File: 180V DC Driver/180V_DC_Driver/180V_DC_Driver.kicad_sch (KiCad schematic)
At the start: 14 parts, among them IC1 TLP250_F_, J1 DC_In, J2 DC_Out, J3 Logic_In, J4 12V_In, Q1 IRFP460PBF

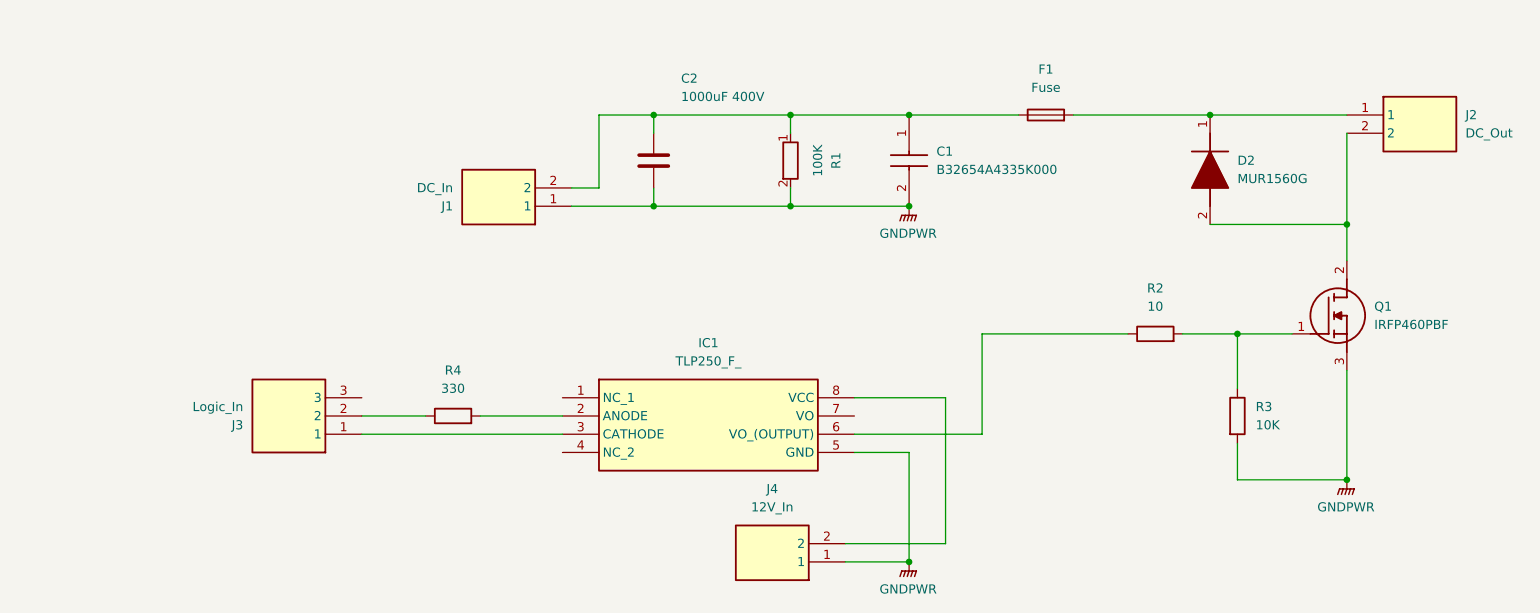
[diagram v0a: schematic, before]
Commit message: c2.06
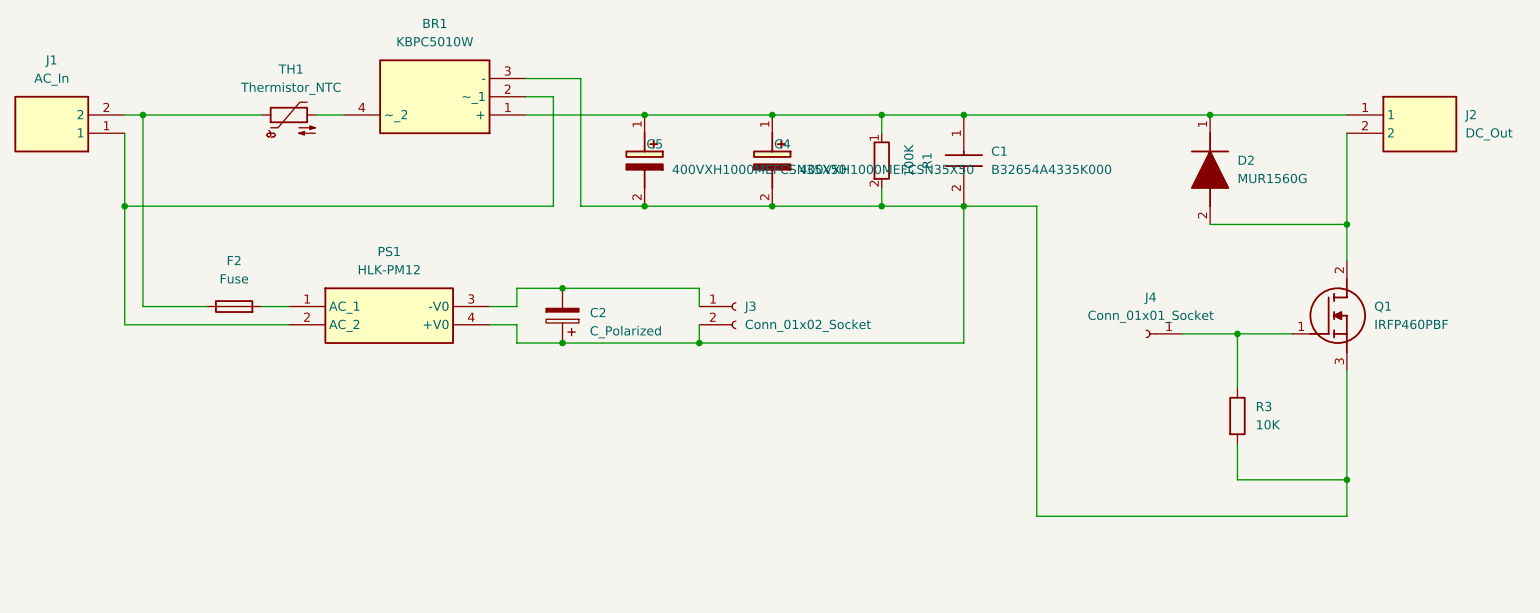
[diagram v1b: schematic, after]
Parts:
- removed C2: 1000uF 400V, symbol Device:C
- removed F1: Fuse, symbol Device:Fuse
- removed IC1: TLP250_F_, DIP762W60P254L966H485Q8N, symbol SamacSys_Parts:TLP250_F_
- removed J3: Logic_In, HDRV3W64P0X254_1X3_762X254X869P, symbol SamacSys_Parts:61300311121
- removed J4: 12V_In, 1935161, symbol SamacSys_Parts:1935161
- removed R2: 10, symbol Device:R
- removed R4: 330, symbol Device:R
- added BR1: KBPC5010W, Diode_THT:Diode_Bridge_28.6x28.6x7.3mm_P18.0mm_P11.6mm, symbol SamacSys_Parts:KBPC5010W
- added C2: C_Polarized, Capacitor_THT:CP_Radial_D6.3mm_P2.50mm, symbol Device:C_Polarized
- added C4, C5: 400VXH1000MEFCSN35X50, Capacitor_THT:CP_Radial_D35.0mm_P10.00mm_SnapIn, symbol SamacSys_Parts:400VXH1000MEFCSN35X50
- added F2: Fuse, Connector_PinHeader_2.54mm:PinHeader_1x02_P2.54mm_Vertical, symbol Device:Fuse
- added J3: Conn_01x02_Socket, Connector_PinHeader_2.54mm:PinHeader_1x02_P2.54mm_Vertical, symbol Connector:Conn_01x02_Socket
- added J4: Conn_01x01_Socket, Connector_PinHeader_2.54mm:PinHeader_1x01_P2.54mm_Vertical, symbol Connector:Conn_01x01_Socket
- added PS1: HLK-PM12, Converter_ACDC:Converter_ACDC_Hi-Link_HLK-PMxx, symbol SamacSys_Parts:HLK-PM12
- added TH1: Thermistor_NTC, Capacitor_THT:C_Disc_D16.0mm_W5.0mm_P10.00mm, symbol Device:Thermistor_NTC
- C1: footprint B32654A4335K000 -> Capacitor_THT:C_Rect_L31.5mm_W20.0mm_P27.50mm_MKS4
- D2: footprint TO533P482X997X1956-2P -> Package_TO_SOT_THT:TO-220-2_Vertical
- J1: value DC_In -> AC_In; footprint 1935161 -> TerminalBlock_Phoenix:TerminalBlock_Phoenix_MKDS-1,5-2-5.08_1x02_P5.08mm_Horizontal
- J2: footprint 1935161 -> TerminalBlock_Phoenix:TerminalBlock_Phoenix_MKDS-1,5-2-5.08_1x02_P5.08mm_Horizontal
- Q1: footprint TO546P531X1558X2511-3P -> Package_TO_SOT_THT:TO-247-3_Vertical
- R1, R3: footprint (none) -> Resistor_THT:R_Axial_DIN0207_L6.3mm_D2.5mm_P10.16mm_Horizontal
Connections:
- net at C1.1, R1.1: now also D2.1 (K), J2.1, BR1.1 (+), C4.1 (+), C5.1 (+); no longer J1.2
- net at Q1.1 (G), R3.1: now also J4.1 (Pin_1)
- net GNDPWR: no longer names the net of C1.2, Q1.3 (S), R1.2, R3.2
- net GNDPWR: now also BR1.3 (-), C2.1, C4.2 (-), C5.2 (-), J3.2 (Pin_2), PS1.4 (+V0); no longer J1.1
- new net: C2.2, J3.1 (Pin_1), PS1.3 (-V0)
- new net: F2.2, PS1.1 (AC_1)
- new net: BR1.2 (~_1), J1.1, PS1.2 (AC_2)
- new net: F2.1, J1.2, TH1.1
- new net: BR1.4 (~_2), TH1.2
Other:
- moved on the sheet: C1, J1, R1

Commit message: c22.06
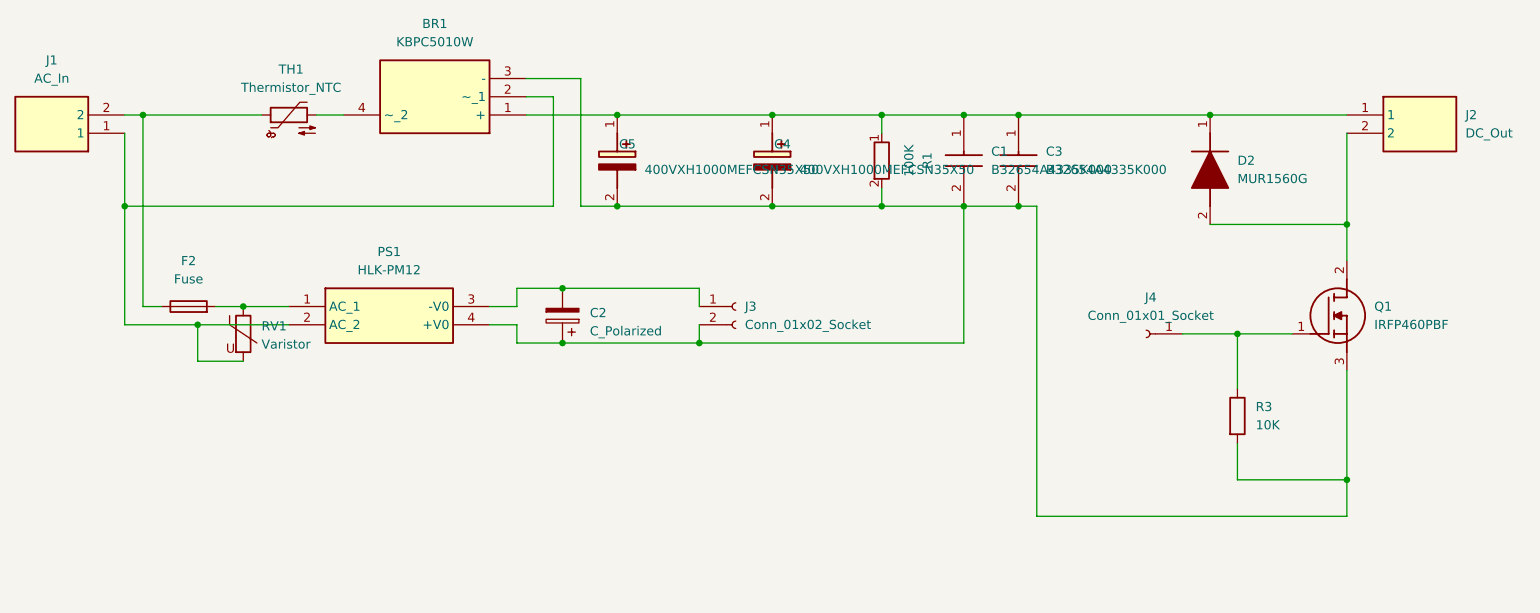
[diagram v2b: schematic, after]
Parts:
- added C3: B32654A4335K000, Capacitor_THT:C_Rect_L31.5mm_W13.0mm_P27.50mm_MKS4, symbol SamacSys_Parts:B32654A4335K000
- added RV1: Varistor, Capacitor_THT:C_Disc_D10.5mm_W5.0mm_P5.00mm, symbol Device:Varistor
- C1: footprint Capacitor_THT:C_Rect_L31.5mm_W20.0mm_P27.50mm_MKS4 -> Capacitor_THT:C_Rect_L31.5mm_W13.0mm_P27.50mm_MKS4
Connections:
- net at BR1.3 (-), C1.2, C2.1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: now also C3.2
- net at F2.2, PS1.1 (AC_1): now also RV1.1
- net at BR1.2 (~_1), J1.1, PS1.2 (AC_2): now also RV1.2
- net at BR1.1 (+), C1.1, C4.1 (+)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: now also C3.1
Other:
- moved on the sheet: C5, F2
